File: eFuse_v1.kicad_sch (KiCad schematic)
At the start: 21 parts, among them J1 Screw_Terminal_01x02, J2 Screw_Terminal_01x02, U2 LD1117S33TR_SOT223

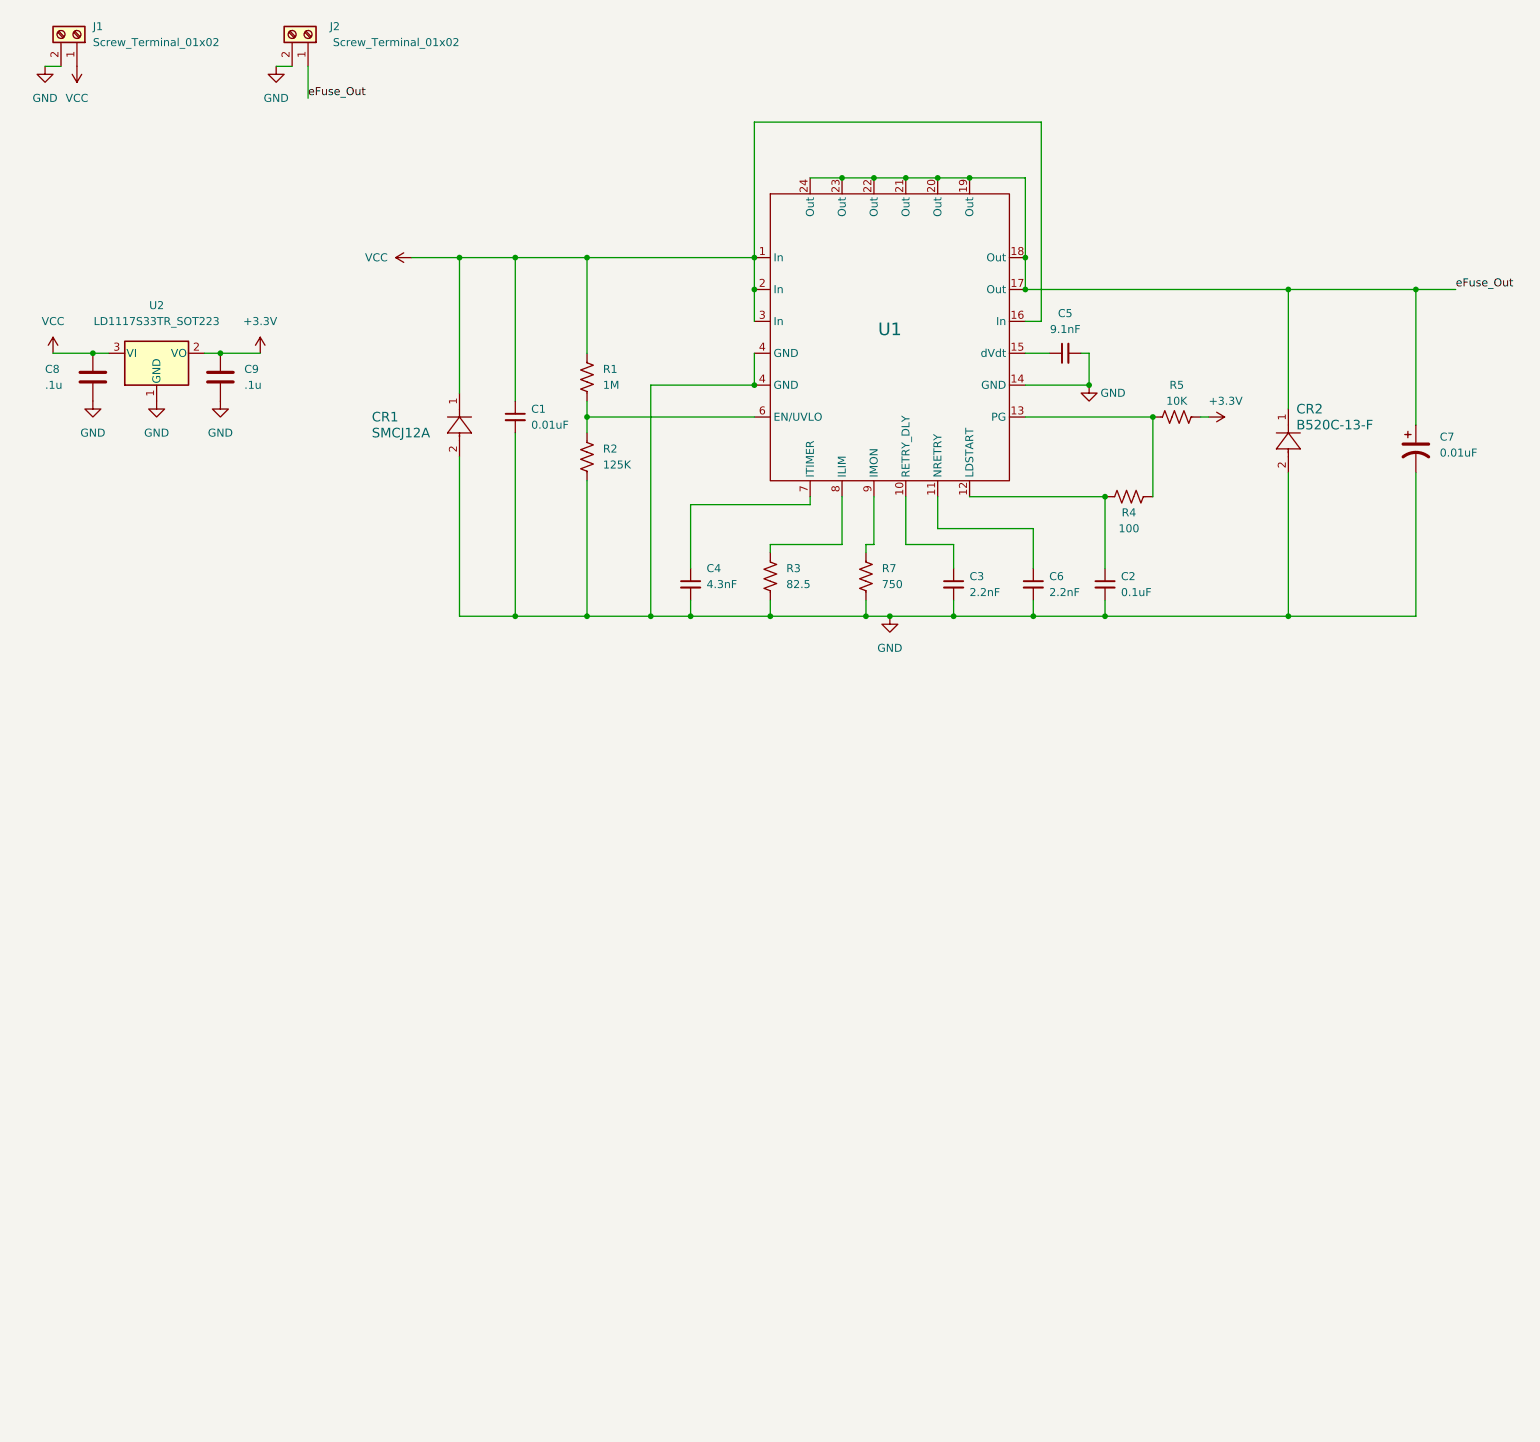
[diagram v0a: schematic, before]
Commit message: updated 3d models
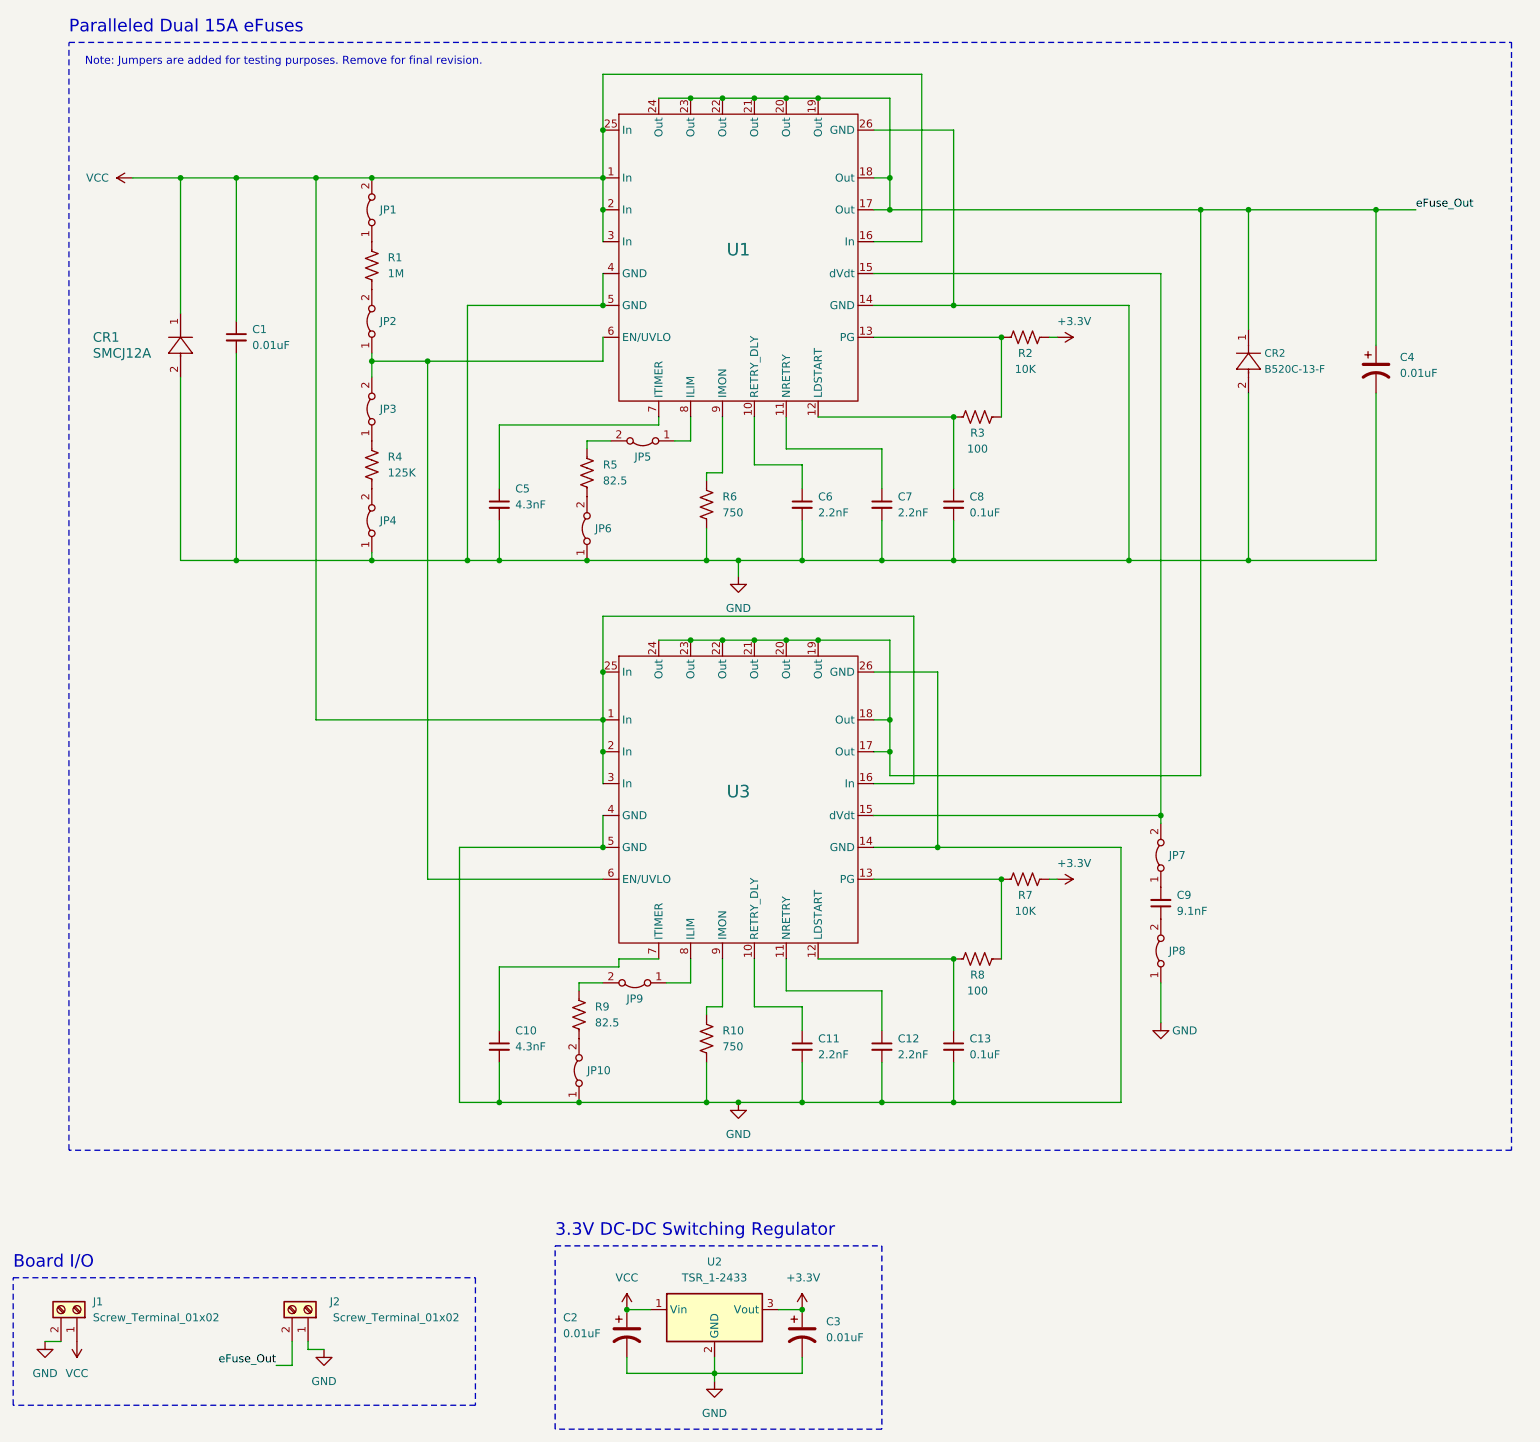
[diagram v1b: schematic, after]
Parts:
- removed C5: 9.1nF, symbol Device:C_Small
- removed C8, C9: .1u, Capacitor_SMD:C_0805_2012Metric, symbol Device:C
- removed U2: LD1117S33TR_SOT223, Package_TO_SOT_SMD:SOT-223-3_TabPin2, symbol Regulator_Linear:LD1117S33TR_SOT223
- added C10: 4.3nF, eFuseLib:CAPC340180_100N_KEM, symbol Device:C_Small
- added C11, C12: 2.2nF, eFuseLib:CAPC10555_55N_KEM, symbol Device:C_Small
- added C13: 0.1uF, eFuseLib:CAPC0603X33N, symbol Device:C_Small
- added C2, C3: 0.01uF, eFuseLib:CAP_GRM033_MUR, symbol Device:C_Polarized_US
- added C9: 9.1nF, eFuseLib:CAPC2012X95N, symbol Device:C_Small
- added JP1, JP10, JP2, JP3, JP4, JP5, JP6, JP7, JP8, JP9: Jumper_2_Bridged, Connector_PinHeader_2.54mm:PinHeader_1x02_P2.54mm_Vertical, symbol Jumper:Jumper_2_Bridged
- added R10: 750, eFuseLib:RESC1005X40N, symbol Device:R_US
- added R7: 10K, eFuseLib:BO_CR0402, symbol Device:R_US
- added R8: 100, eFuseLib:RC0402N_YAG, symbol Device:R_US
- added R9: 82.5, eFuseLib:YAG_R0402_YAG, symbol Device:R_US
- added U2: TSR_1-2433, Converter_DCDC:Converter_DCDC_TRACO_TSR-1_THT, symbol Regulator_Switching:TSR_1-2433
- added U3: ~, eFuseLib:RGE24_2P5XP85X1P45_TEX, symbol eFuseLib:TPS259823LNRGET
- C1: footprint (none) -> eFuseLib:CAP_GRM033_MUR
- C4: renamed from C7; footprint (none) -> eFuseLib:CAP_GRM033_MUR
- C5: renamed from C4; footprint (none) -> eFuseLib:CAPC340180_100N_KEM
- C6: renamed from C3; footprint (none) -> eFuseLib:CAPC10555_55N_KEM
- C7: renamed from C6; footprint (none) -> eFuseLib:CAPC10555_55N_KEM
- C8: renamed from C2; footprint (none) -> eFuseLib:CAPC0603X33N
- CR1: footprint SMCJSeries_LTF -> Diode_SMD:D_SMC
- CR2: footprint SMC_DIO -> Diode_SMD:D_SMC
- J1, J2: footprint Connector_PinHeader_2.54mm:PinHeader_1x02_P2.54mm_Vertical -> TerminalBlock_Phoenix:TerminalBlock_Phoenix_PT-1,5-2-5.0-H_1x02_P5.00mm_Horizontal
- R1: footprint (none) -> eFuseLib:RES_ERJ2RKF1004X
- R2: renamed from R5; footprint (none) -> eFuseLib:BO_CR0402
- R3: renamed from R4; footprint (none) -> eFuseLib:RC0402N_YAG
- R4: renamed from R2; footprint (none) -> eFuseLib:RESC1005X35N
- R5: renamed from R3; footprint (none) -> eFuseLib:YAG_R0402_YAG
- R6: renamed from R7; footprint (none) -> eFuseLib:RESC1005X40N
- U1: footprint Package_DFN_QFN:QFN-24-1EP_4x4mm_P0.5mm_EP2.7x2.6mm -> eFuseLib:RGE24_2P5XP85X1P45_TEX
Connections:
- net +3.3V: now also C3.1, R7.2, U2.3 (Vout)
- net GND: now also J2.1 (Pin_1), U1.26 (GND), U1.5 (GND), C10.2, C11.2, C12.2, C13.2, C2.2, C3.2, JP10.1 (A), JP4.1 (A), JP6.1 (A), JP8.1 (A), R10.2, U2.2 (GND), U3.14 (GND), U3.26 (GND), U3.4 (GND), U3.5 (GND); no longer J2.2 (Pin_2), R4.2, R5.2
- net VCC: now also U1.25 (In), C2.1, JP1.2 (B), U2.1 (Vin), U3.1 (In), U3.16 (In), U3.2 (In), U3.25 (In), U3.3 (In); no longer R1.1
- net eFuse_Out: now also J2.2 (Pin_2), U3.17 (Out), U3.18 (Out), U3.19 (Out), U3.20 (Out), U3.21 (Out), U3.22 (Out), U3.23 (Out), U3.24 (Out); no longer J2.1 (Pin_1)
- net at U1.15 (dVdt): now also JP7.2 (B), U3.15 (dVdt)
- net at U1.8 (ILIM): now also JP5.1 (A); no longer R5.1
- new net: JP1.1 (A), R1.1
- new net: JP2.2 (B), R1.2
- new net: C12.1, U3.11 (NRETRY)
- new net: JP4.2 (B), R4.2
- new net: R7.1, R8.2, U3.13 (PG)
- new net: JP2.1 (A), JP3.2 (B), U1.6 (EN/UVLO), U3.6 (EN/UVLO)
- new net: JP6.2 (B), R5.2
- new net: C9.1, JP8.2 (B)
- new net: JP10.2 (B), R9.2
- new net: C11.1, U3.10 (RETRY_DLY)
- new net: C13.1, R8.1, U3.12 (LDSTART)
- new net: C10.1, U3.7 (ITIMER)
- new net: JP9.1 (A), U3.8 (ILIM)
- new net: R10.1, U3.9 (IMON)
- new net: C9.2, JP7.1 (A)
- new net: JP5.2 (B), R5.1
- new net: JP3.1 (A), R4.1
- new net: JP9.2 (B), R9.1
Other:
- note added: "3.3V DC-DC Switching Regulator"
- note added: "Board I/O"
- note added: "Note: Jumpers are added for testing purposes. Remove for final revision."
- note added: "Paralleled Dual 15A eFuses"
- title: eFuse -> Parallel 15A eFuse
- moved on the sheet: C1, C4, C5, C6, C7, C8, CR1, J1, J2, R1, R2, R3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
